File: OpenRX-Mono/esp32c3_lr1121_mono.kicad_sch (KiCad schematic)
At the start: 61 parts, among them J1 Conn_Coaxial_Small, T1 0900PC16J0042001E, U1 ESP32-C3, U2 TLV75533PDQNR, U3 LR1121IMLTRT, U4 RFX2401C, U5 SKY13373-460LF, X1 CJ17-400001010B20

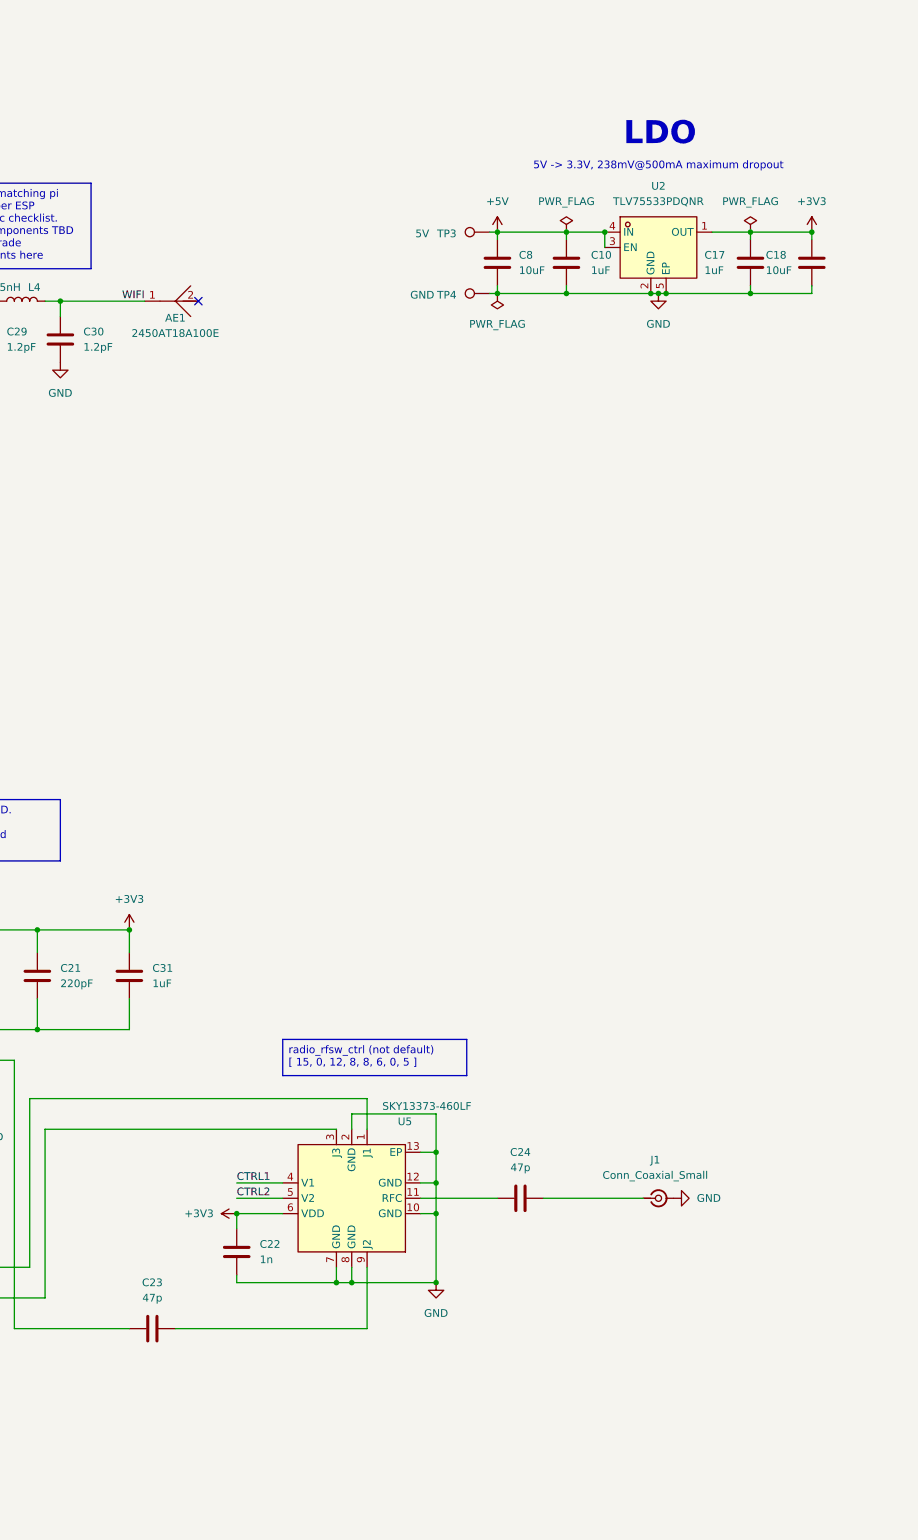
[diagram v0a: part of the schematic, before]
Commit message: annotate
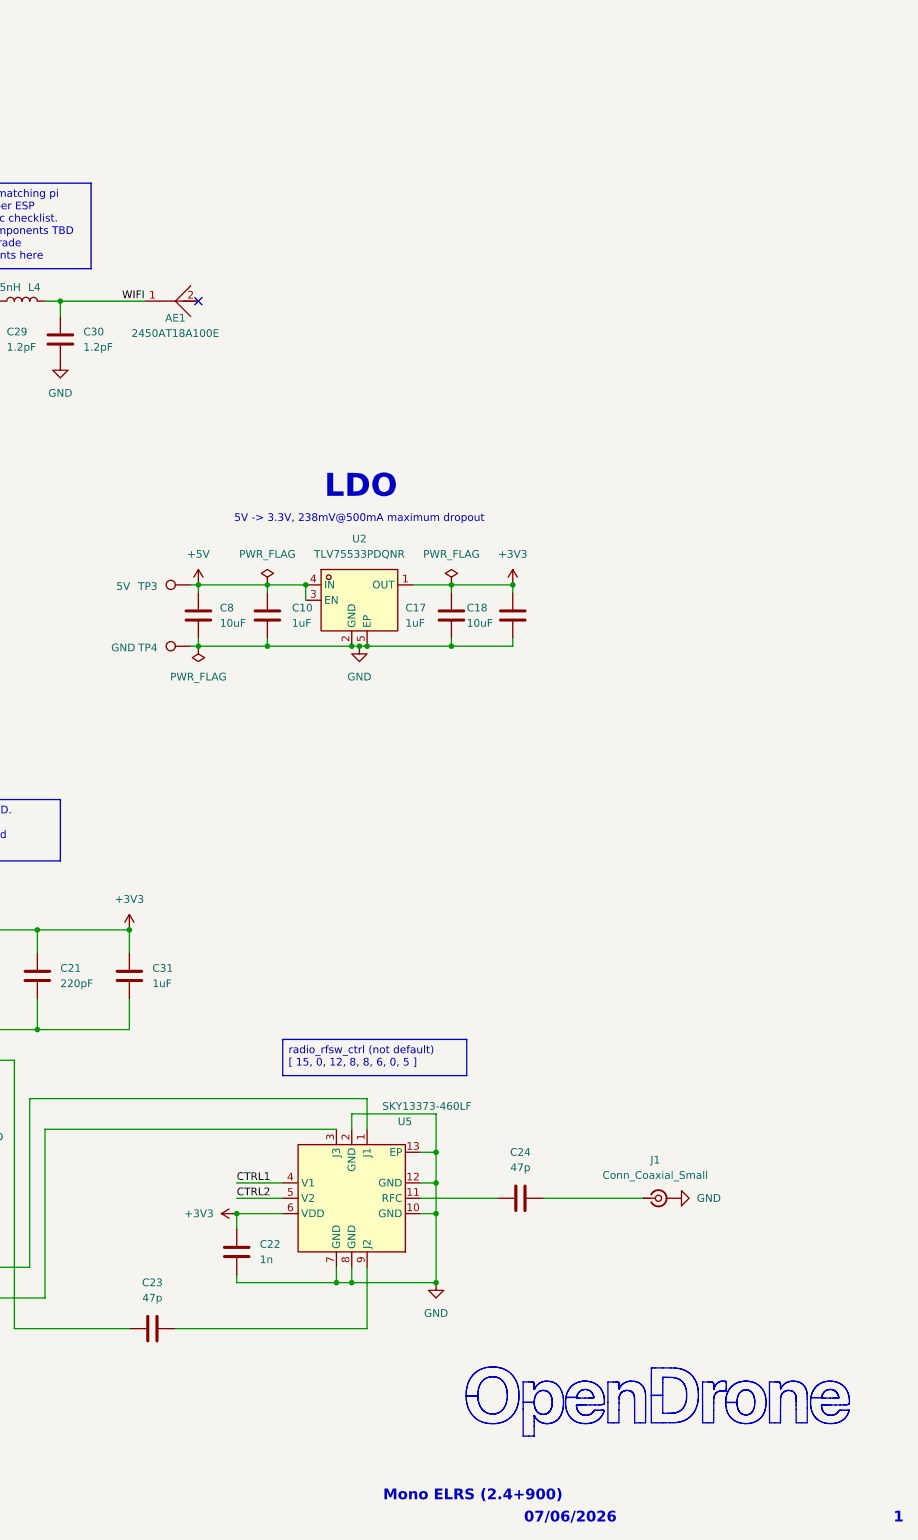
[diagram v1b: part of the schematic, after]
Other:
- note added: "07/06/2026"
- note added: "1"
- note added: "Mono ELRS (2.4+900)"
- moved on the sheet: C10, C17, C18, C8, TP3, TP4, U2
